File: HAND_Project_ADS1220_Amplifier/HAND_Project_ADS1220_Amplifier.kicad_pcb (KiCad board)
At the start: 2 copper layers, 30.5 x 38.1 mm, 17 parts, among them J2 Conn_01x05_Pin, J7 Conn_01x04_Pin

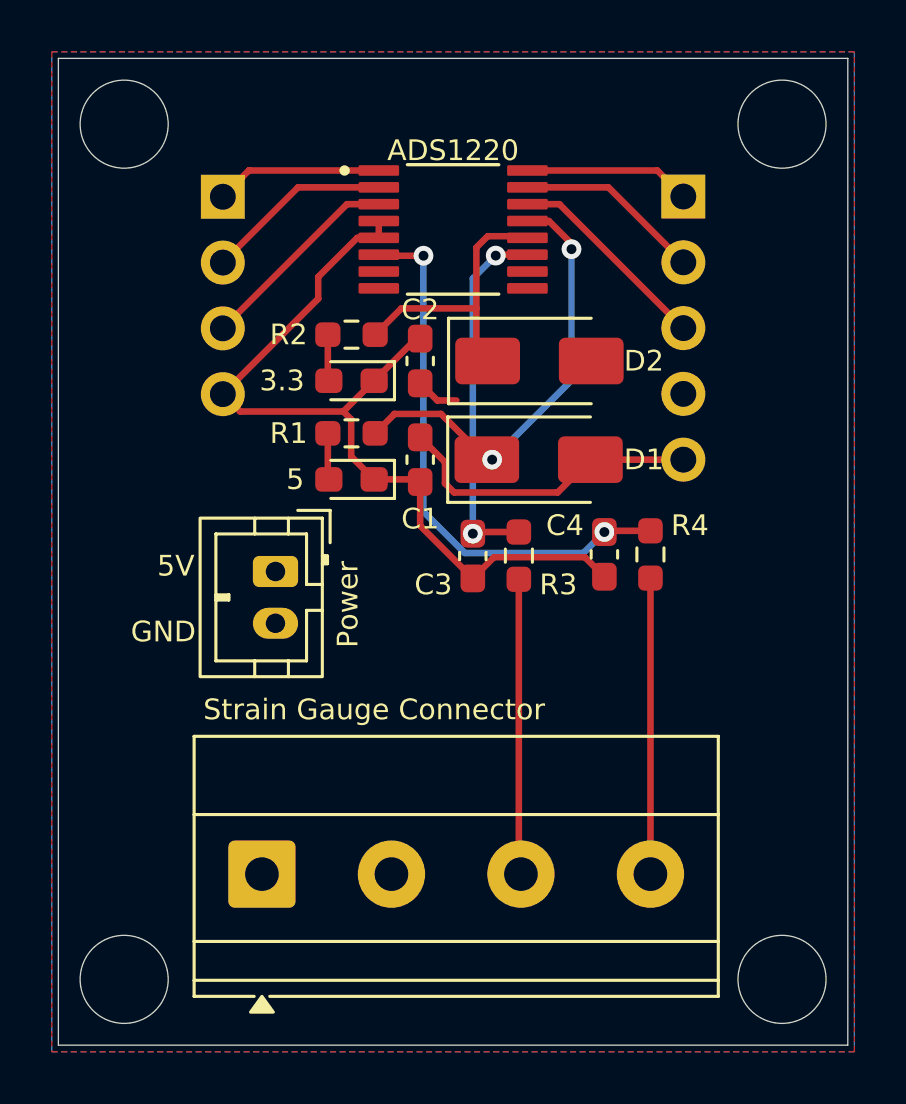
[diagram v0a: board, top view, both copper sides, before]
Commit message: Final touches
matched footprints with yuchan's PCB
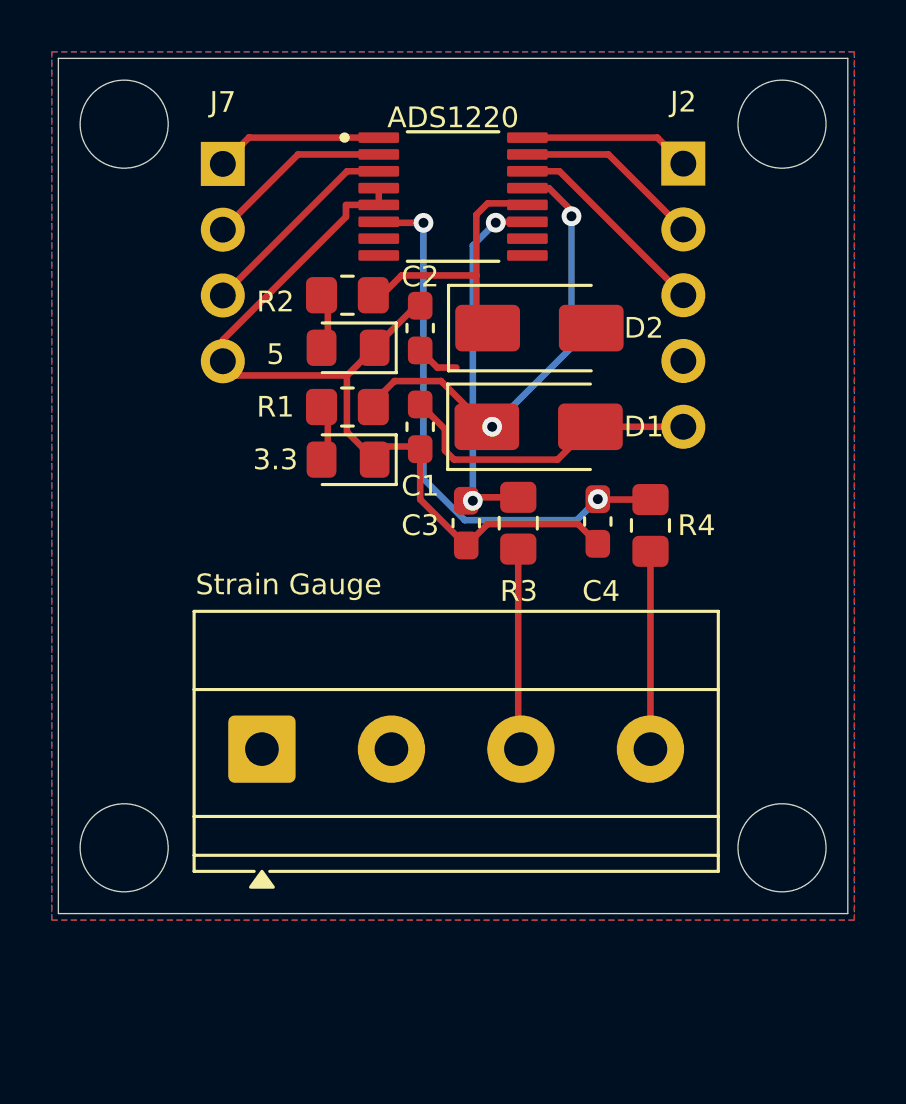
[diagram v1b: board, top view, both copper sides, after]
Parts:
- removed Power: Conn_01x02_Pin, Connector_JST:JST_PH_B2B-PH-K_1x02_P2.00mm_Vertical
- 3.3: renamed from 5; footprint LED_SMD:LED_0603_1608Metric_Pad1.05x0.95mm_HandSolder -> LED_SMD:LED_0805_2012Metric_Pad1.15x1.40mm_HandSolder
- 5: renamed from 3.3; footprint LED_SMD:LED_0603_1608Metric_Pad1.05x0.95mm_HandSolder -> LED_SMD:LED_0805_2012Metric_Pad1.15x1.40mm_HandSolder
- C3, C4: value 15 nF -> 10nF
- R1, R2: value 330 -> 360; footprint Resistor_SMD:R_0603_1608Metric_Pad0.98x0.95mm_HandSolder -> Resistor_SMD:R_0805_2012Metric_Pad1.20x1.40mm_HandSolder
- R3, R4: value 10k -> 16k; footprint Resistor_SMD:R_0603_1608Metric_Pad0.98x0.95mm_HandSolder -> Resistor_SMD:R_0805_2012Metric_Pad1.20x1.40mm_HandSolder
- Strain Gauge: renamed from Strain Gauge Connector
- moved Strain Gauge 4.83 mm to (131.1, 91.4)
- moved R2 1.53 mm to (134.3, 73.9)
- moved C4 1.30 mm to (144.0, 82.7)
- moved C3 1.30 mm to (138.9, 82.7)
- moved 5 1.28 mm to (134.4, 75.9)
- moved J7 1.27 mm to (129.5, 68.8)
- moved ADS1220 1.27 mm to (138.4, 70.1)
- moved C1 1.27 mm to (137.2, 79.0)
- moved C2 1.27 mm to (137.2, 75.2)
- moved D1 1.27 mm to (141.7, 79.0)
- moved D2 1.27 mm to (141.8, 75.2)
- moved J2 1.27 mm to (147.3, 68.8)
- moved R3 1.25 mm to (140.9, 82.7)
- moved R4 1.12 mm to (146.1, 82.8)
- moved R1 1.03 mm to (134.3, 78.2)
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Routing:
- net Net-(J1-Pin_4): track 11.4 -> 7.64 mm
- net Net-(J1-Pin_3): track 11.4 -> 7.91 mm
- net GND: track 34.7 -> 35.2 mm
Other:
- board size 30.5 x 38.1 mm -> 30.5 x 33 mm
- board text removed: "5V"
- board text removed: "GND"
